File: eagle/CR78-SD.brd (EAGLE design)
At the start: 100 x 80 mm, 46 parts, among them Q1 2N3904, Q2 2N3904, Q3 2N3904, Q4 2N3904, Q7 2N3904

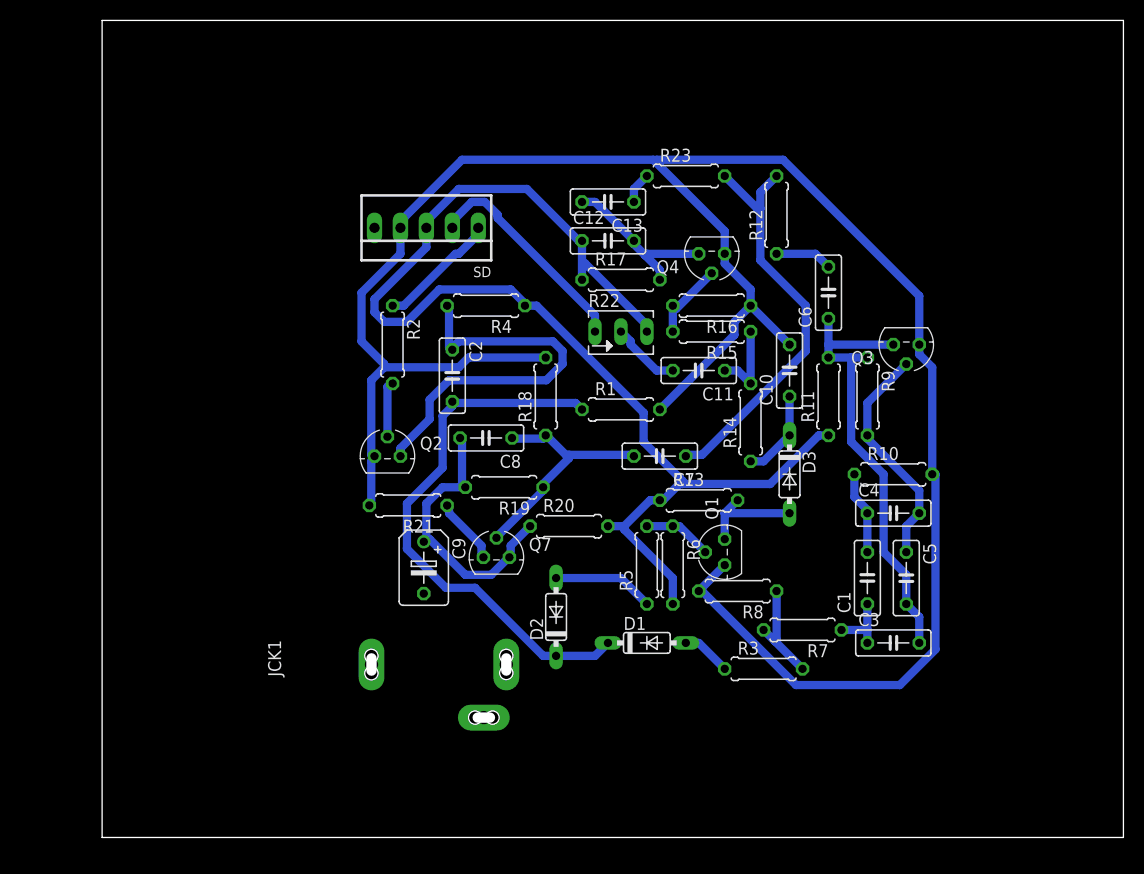
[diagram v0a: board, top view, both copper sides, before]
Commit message: routed and cutout
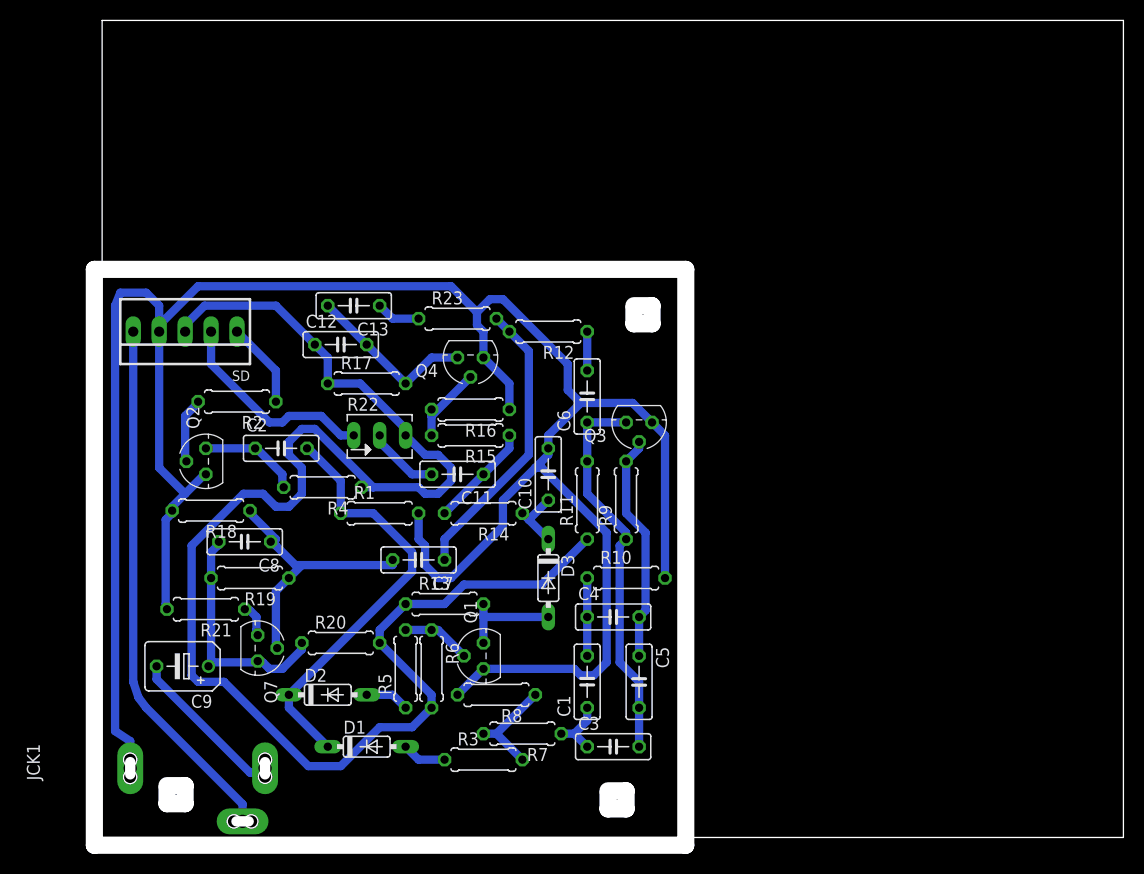
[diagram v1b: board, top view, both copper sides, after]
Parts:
- moved R18 34.6 mm to (10.7, 32.0), turned to 180 degrees
- moved C1 29.3 mm to (47.5, 15.2)
- moved C3 29.3 mm to (50.0, 8.89)
- moved C4 29.3 mm to (50.0, 21.6)
- moved D1 29.3 mm to (25.9, 8.89)
- moved R7 29.3 mm to (41.1, 10.2)
- moved R3 28.8 mm to (37.3, 7.62)
- moved C12 28.1 mm to (23.4, 48.3)
- moved R10 28.1 mm to (51.3, 25.4)
- moved C5 28.1 mm to (52.6, 15.2)
- moved R14 27.6 mm to (37.3, 31.8), turned to 180 degrees
- moved Q3 27.2 mm to (52.6, 40.6)
- moved R13 26.9 mm to (33.5, 22.9)
- moved C13 26.9 mm to (24.6, 52.1)
- moved R17 26.9 mm to (25.9, 44.5)
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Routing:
- net N$7: track 0.00 -> 52.2 mm
- net +12V: track 119.5 -> 153.4 mm
- net GND: track 211.1 -> 240.9 mm
- net N$46: track 38.8 -> 9.94 mm
- net N$19: track 0.00 -> 15.9 mm
- net N$13: track 40.5 -> 28.4 mm
- net N$2: track 53.9 -> 42.0 mm
- net N$5: track 44.7 -> 38.2 mm
- net N$3: track 9.94 -> 4.34 mm
- net N$16: track 27.9 -> 23.2 mm
- net N$11: track 11.9 -> 8.44 mm
- net N$15: track 6.58 -> 3.22 mm
- net N$18: track 24.1 -> 27.0 mm
- net N$17: track 8.67 -> 6.29 mm
- net N$20: track 8.15 -> 10.3 mm
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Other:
- board size 100 x 80 mm -> 100.8 x 80.8 mm
